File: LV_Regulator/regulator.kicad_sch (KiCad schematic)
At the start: 11 parts, among them U1 BQ25858QWRRVRQ1, U2 CSD19506KTT, U3 CSD19506KTT, U4 CSD19506KTT, U5 CSD19506KTT

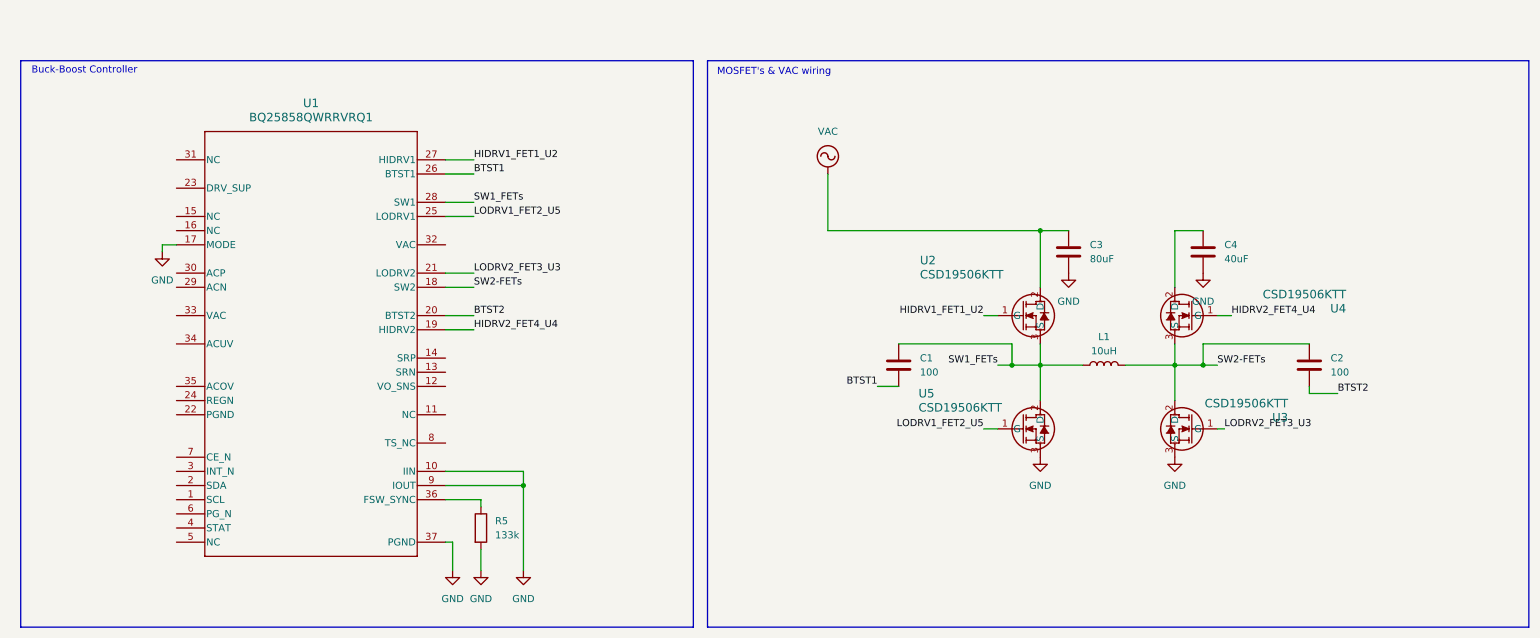
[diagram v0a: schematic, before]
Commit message: Fixed last commit
Fixed all mistakes from the last push
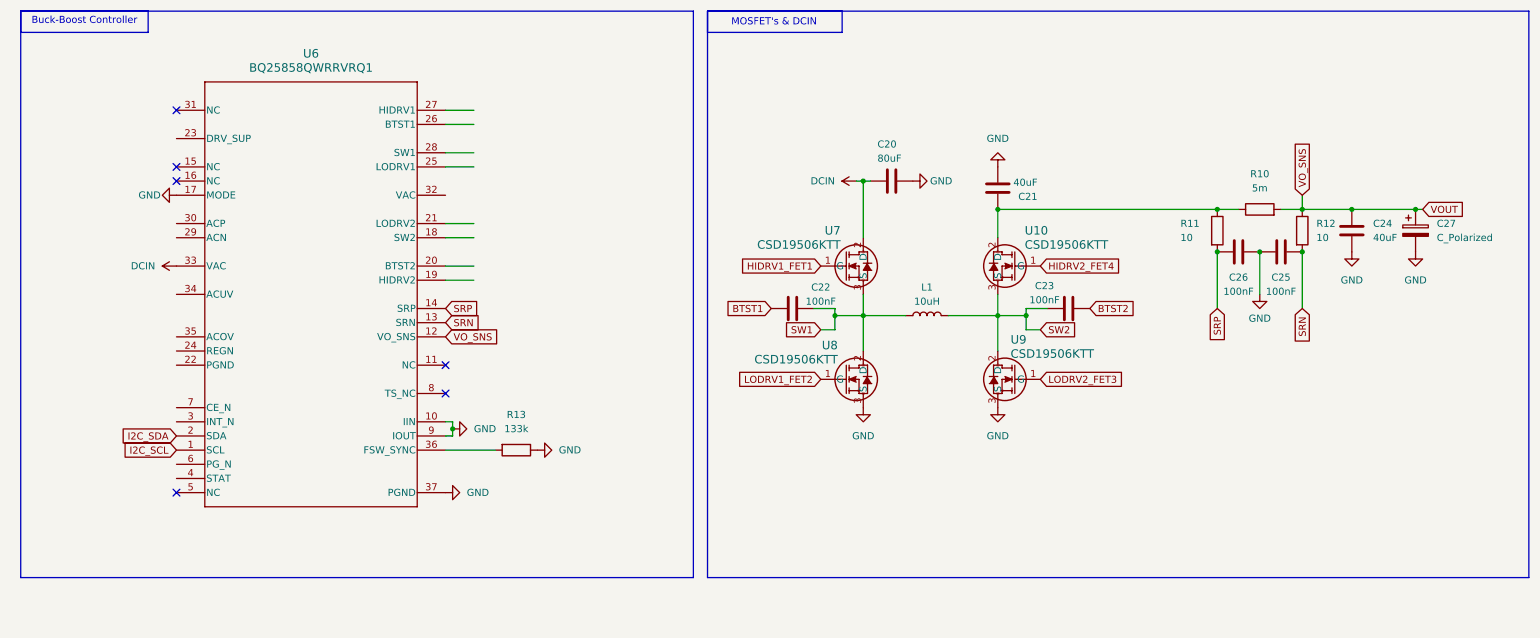
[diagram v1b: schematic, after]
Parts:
- removed C1, C2: 100, symbol Device:C
- removed C3: 80uF, symbol Device:C
- removed C4: 40uF, symbol Device:C
- added C20: 80uF, symbol Device:C
- added C21, C24: 40uF, symbol Device:C
- added C22, C23, C25, C26: 100nF, symbol Device:C
- added C27: C_Polarized, symbol Device:C_Polarized
- added R10: 5m, symbol Device:R
- added R11, R12: 10, symbol Device:R
- renumbered R5 to R13, U4 to U10, U1 to U6, U2 to U7, U5 to U8, U3 to U9
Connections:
- net VAC is gone; now on net DCIN: U7.2 (D)
- net BTST2: now also C23.1; no longer U6.20 (BTST2)
- net GND: now also R13.1, C20.2, C21.2, C24.2, C25.1, C26.2, C27.2; no longer R13.2
- net at U6.26 (BTST1): no longer names the net of U6.26 (BTST1)
- net at U10.2 (D): now also C21.1, R10.1, R11.1
- net at U6.36 (FSW_SYNC): now also R13.2; no longer R13.1
- net I2C_SCL: now reaches U6.1 (SCL)
- net VOUT: now reaches U6.12 (VO_SNS)
- net VOUT: now also C24.1, C27.1, R10.2, R12.1
- net SRN: now reaches U6.13 (SRN)
- net SRN: now also C25.2, R12.2
- net SRP: now reaches U6.14 (SRP)
- net SRP: now also C26.1, R11.2
- net I2C_SDA: now reaches U6.2 (SDA)
- net DCIN: now reaches U6.33 (VAC)
- net DCIN: now also C20.1
- net HIDRV1_FET1_U2: no longer names the net of U6.27 (HIDRV1)
- net HIDRV1_FET1_U2: no longer U7.1 (G)
- net HIDRV2_FET4_U4: no longer names the net of U6.19 (HIDRV2)
- net HIDRV2_FET4_U4: no longer U10.1 (G)
- net LODRV1_FET2_U5: no longer names the net of U6.25 (LODRV1)
- net LODRV1_FET2_U5: no longer U8.1 (G)
- net LODRV2_FET3_U3: no longer names the net of U6.21 (LODRV2)
- net LODRV2_FET3_U3: no longer U9.1 (G)
- net SW1_FETs renamed SW1
- net SW1: now also C22.2; no longer U6.28 (SW1)
- net SW2-FETs renamed SW2
- net SW2: now also C23.2; no longer U6.18 (SW2)
- new net BTST1: C22.1
- new net HIDRV1_FET1: U7.1 (G)
- new net HIDRV2_FET4: U10.1 (G)
- new net LODRV1_FET2: U8.1 (G)
- new net LODRV2_FET3: U9.1 (G)
- no-connect marks 0 -> 6
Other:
- note added: "MOSFET's & DCIN"
- note removed: "MOSFET's & VAC wiring"
- moved on the sheet: R13, U10, U6, U7, U8, U9
